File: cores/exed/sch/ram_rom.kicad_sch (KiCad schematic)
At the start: 6 parts

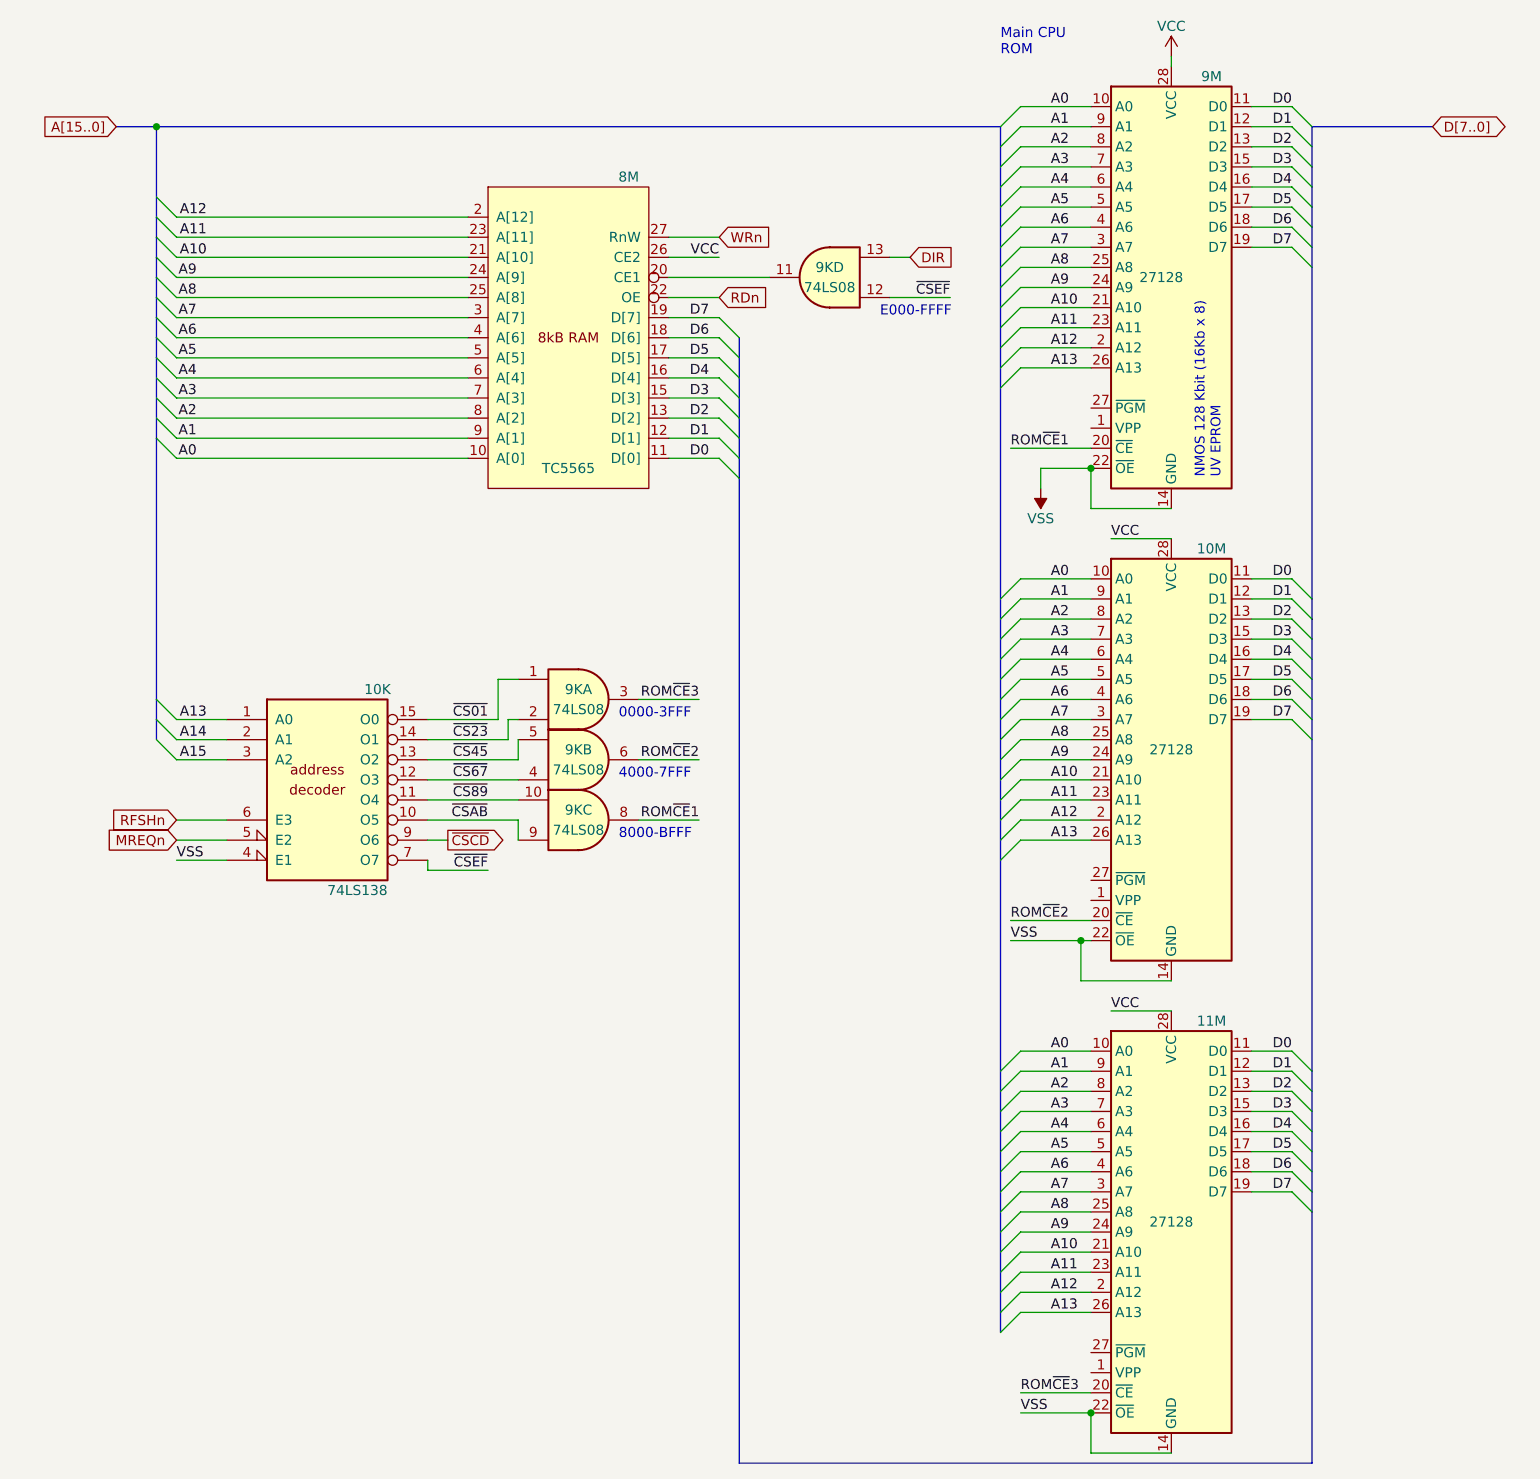
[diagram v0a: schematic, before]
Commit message: exed_cre_wip
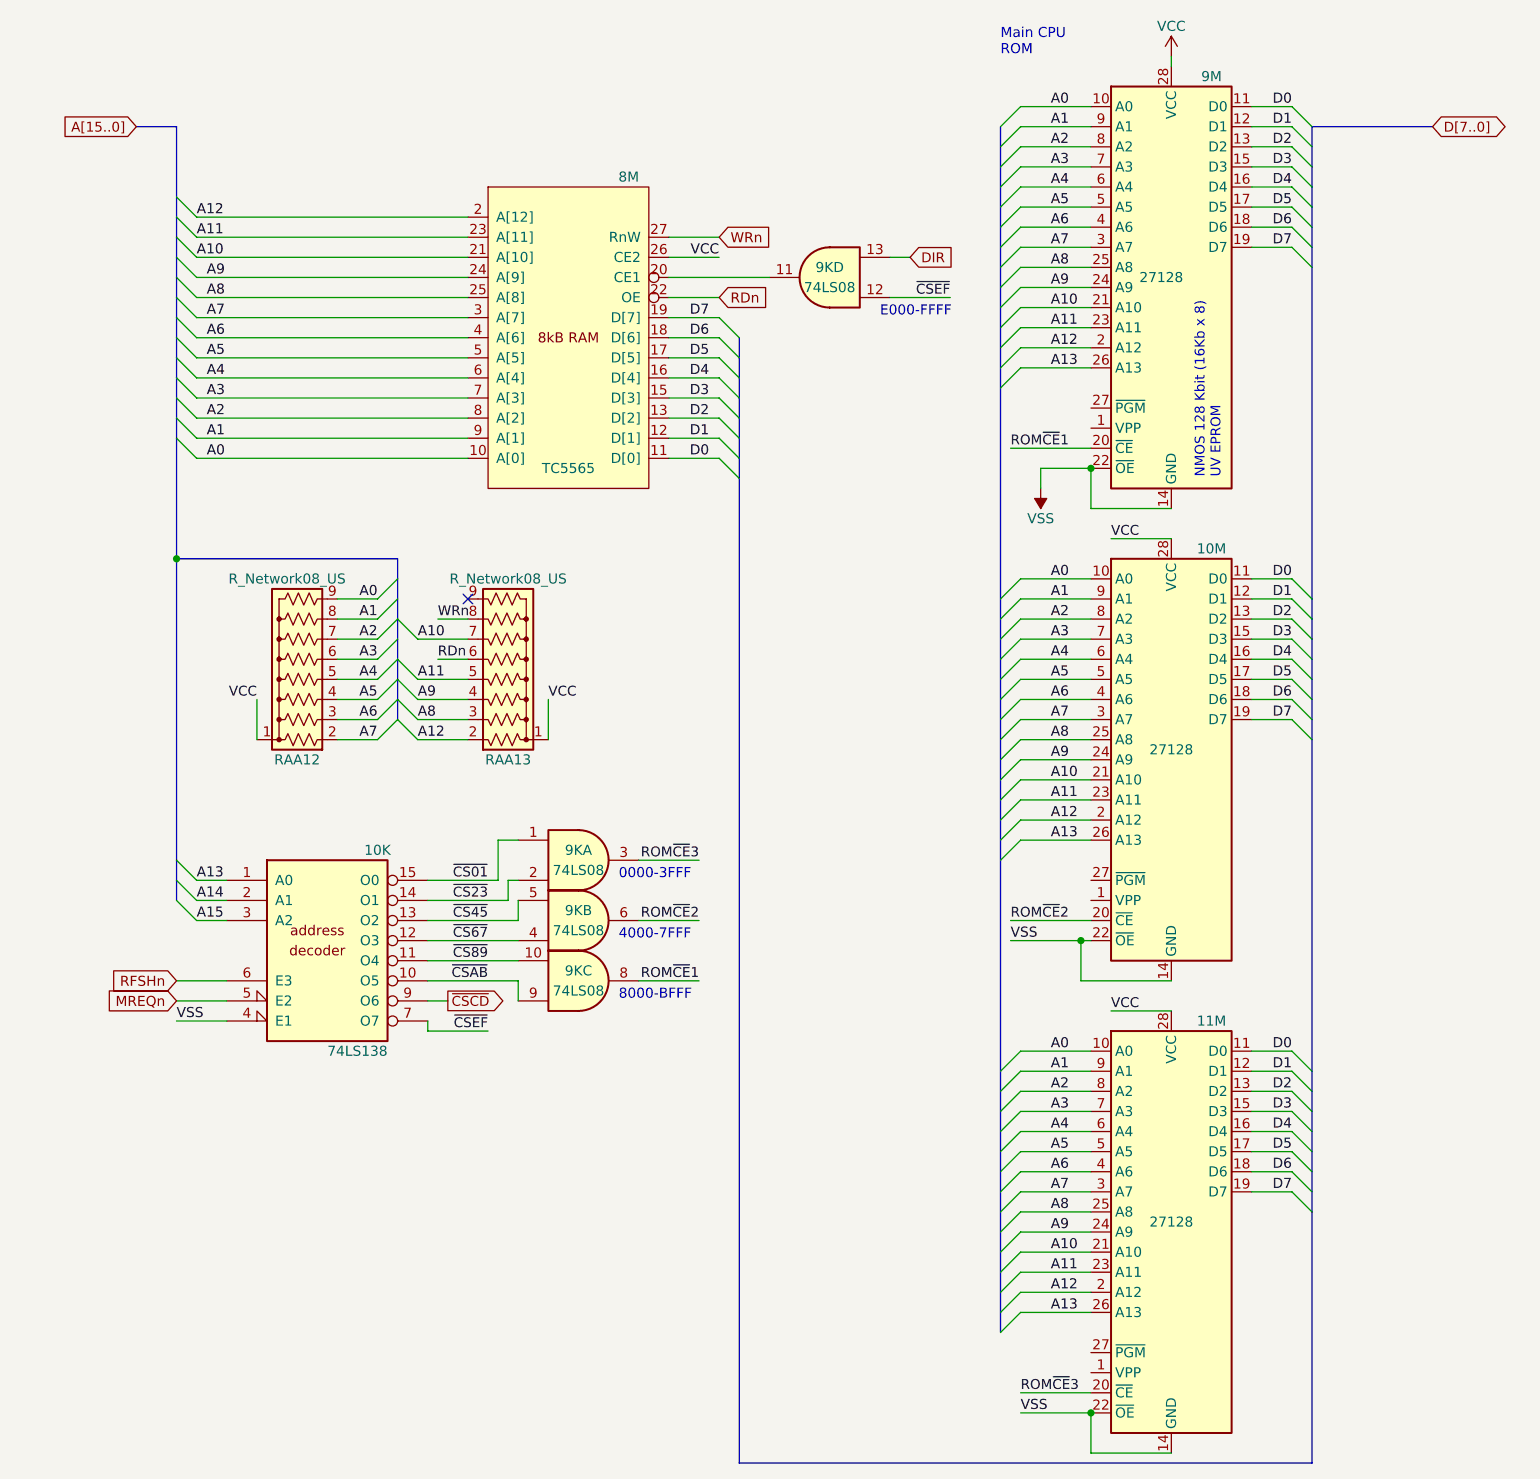
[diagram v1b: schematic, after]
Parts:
- added RAA12, RAA13: R_Network08_US, Resistor_THT:R_Array_SIP9, symbol Device:R_Network08_US
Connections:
- net A0: now also RAA12.9 (R8)
- net A1: now also RAA12.8 (R7)
- net A10: now also RAA13.7 (R6)
- net A11: now also RAA13.5 (R4)
- net A12: now also RAA13.2 (R1)
- net A2: now also RAA12.7 (R6)
- net A3: now also RAA12.6 (R5)
- net A4: now also RAA12.5 (R4)
- net A5: now also RAA12.4 (R3)
- net A6: now also RAA12.3 (R2)
- net A7: now also RAA12.2 (R1)
- net A8: now also RAA13.3 (R2)
- net A9: now also RAA13.4 (R3)
- net RDn: now also RAA13.6 (R5)
- net VCC: now also RAA12.1 (common), RAA13.1 (common)
- net WRn: now also RAA13.8 (R7)
- no-connect marks 0 -> 1
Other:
- moved on the sheet: 10K, 9KA, 9KB, 9KC
